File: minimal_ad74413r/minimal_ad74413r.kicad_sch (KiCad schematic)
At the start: 60 parts, among them J1 FW-02-03-G-D-085-155, J2 FW-02-03-G-D-085-155, J3 FW-02-03-G-D-085-155, J4 FW-02-03-G-D-085-155, J5 FW-02-03-G-D-085-155, J6 FW-02-03-G-D-085-155, J7 FW-14-03-G-D-085-155, U1 AD74413RBCPZ

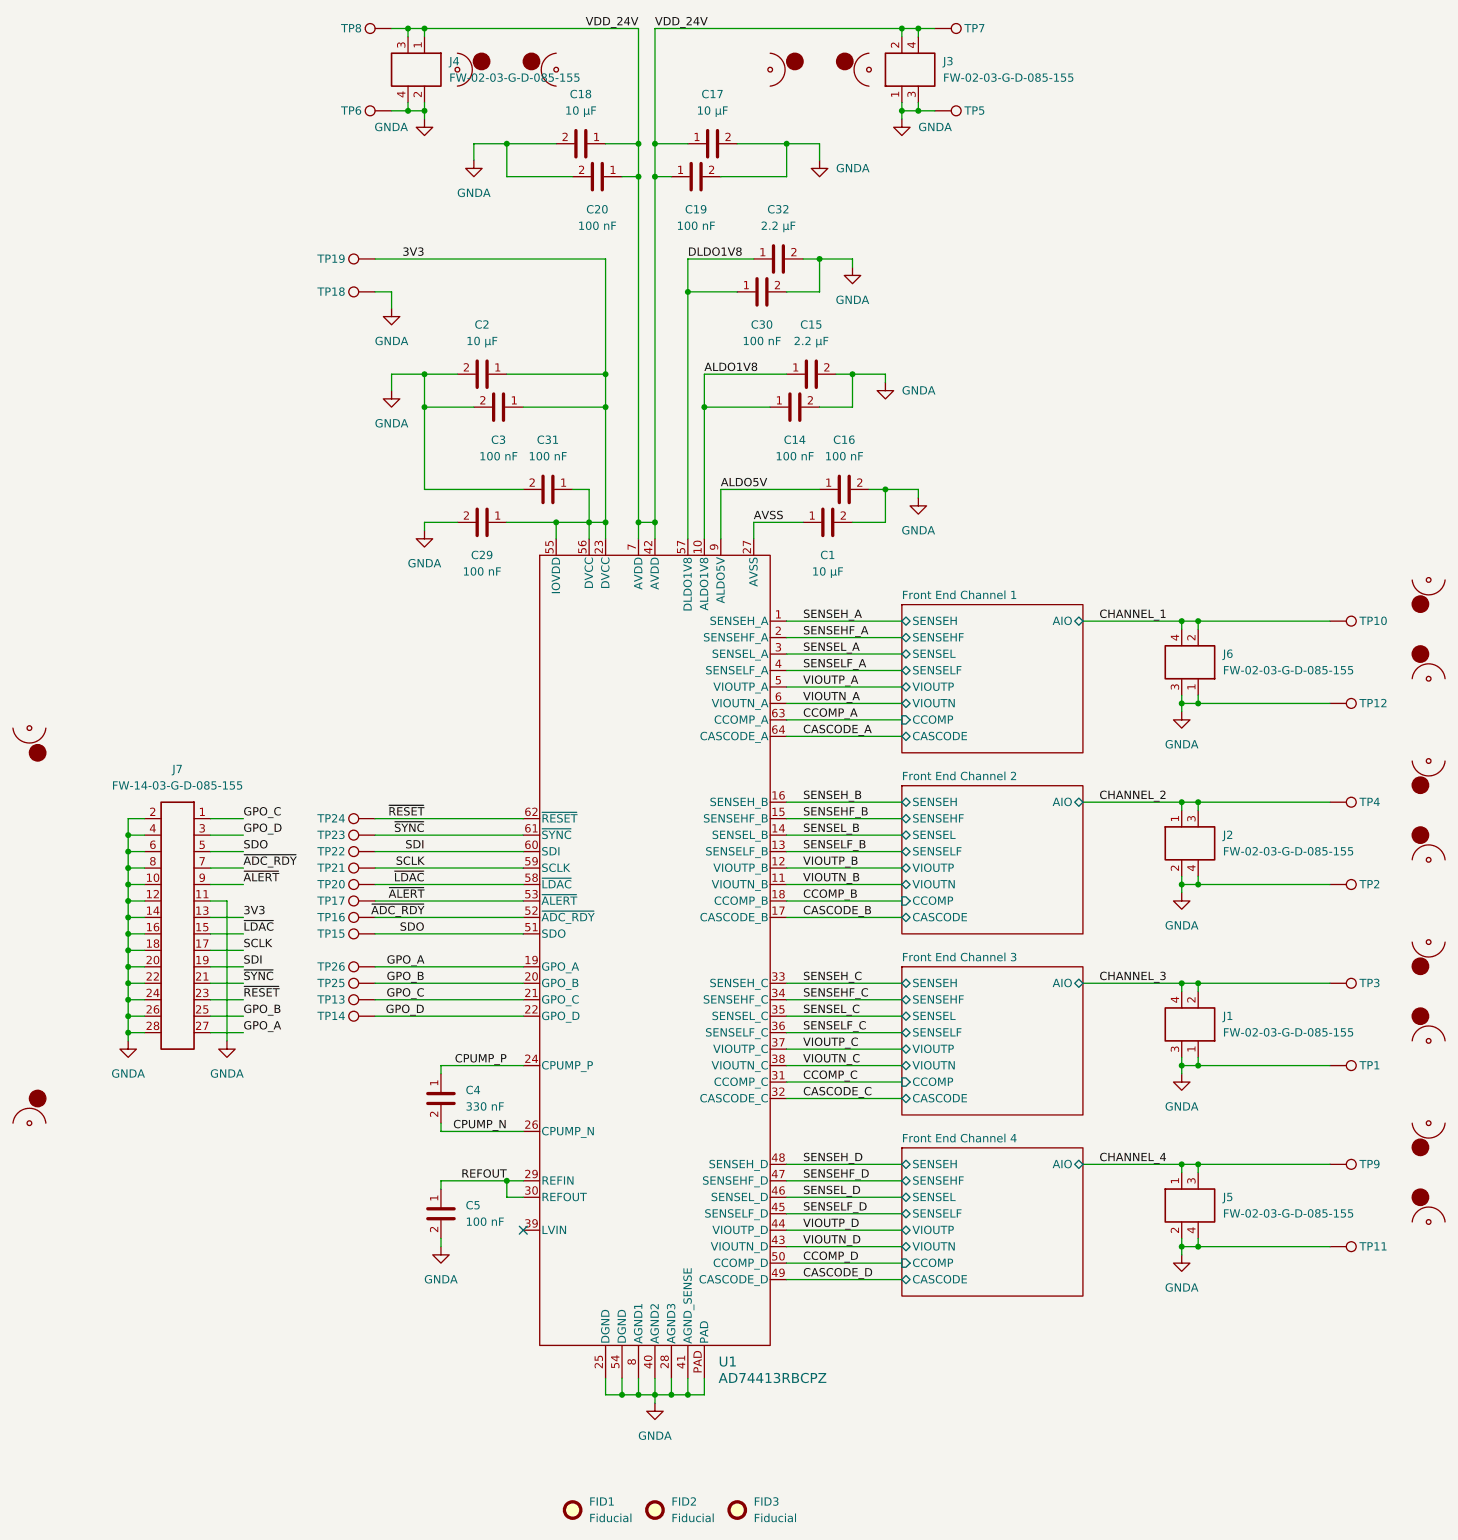
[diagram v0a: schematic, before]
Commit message: Switch to KiCad 9
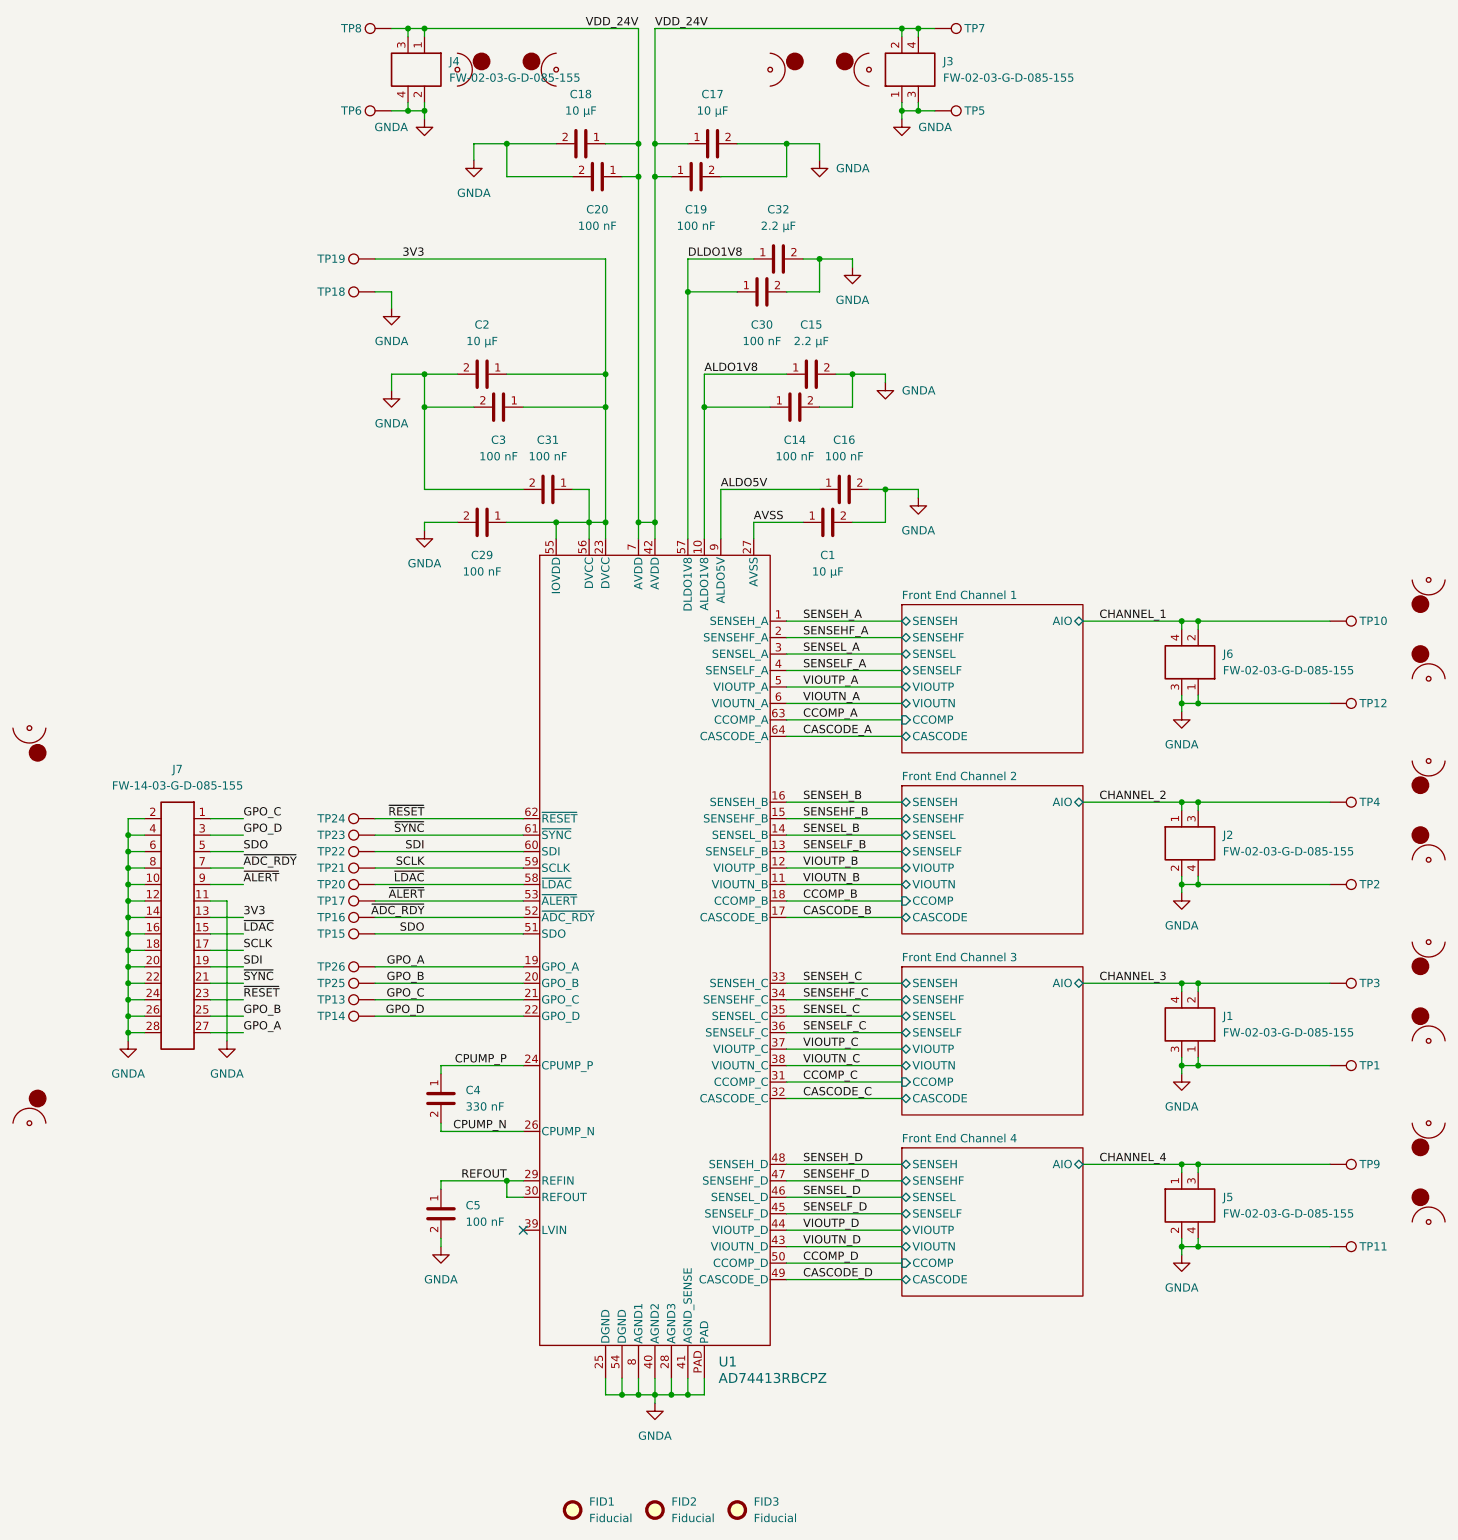
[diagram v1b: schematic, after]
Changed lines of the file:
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@@
 (kicad_sch
-	(version 20231120)
+	(version 20250114)
 	(generator "eeschema")
-	(generator_version "8.0")
+	(generator_version "9.0")
 	(paper "A3")
 	(junction
@@
 		(at 241.3 170.18)
 		(size 27.94 22.86)
+		(exclude_from_sim no)
+		(in_bom yes)
+		(on_board yes)
+		(dnp no)
 		(fields_autoplaced yes)
 		(stroke
@@
 		(at 241.3 114.3)
 		(size 27.94 22.86)
+		(exclude_from_sim no)
+		(in_bom yes)
+		(on_board yes)
+		(dnp no)
 		(fields_autoplaced yes)
 		(stroke
@@
 		(at 241.3 198.12)
 		(size 27.94 22.86)
+		(exclude_from_sim no)
+		(in_bom yes)
+		(on_board yes)
+		(dnp no)
 		(fields_autoplaced yes)
 		(stroke
@@
 		(at 241.3 142.24)
 		(size 27.94 22.86)
+		(exclude_from_sim no)
+		(in_bom yes)
+		(on_board yes)
+		(dnp no)
 		(fields_autoplaced yes)
 		(stroke
@@
 		)
 	)
+	(embedded_fonts no)
 )
